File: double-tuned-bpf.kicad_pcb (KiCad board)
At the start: 2 copper layers, 92 x 71 mm, 96 parts, among them J1 PCB_SMA_EDGE, J2 PCB_SMA_EDGE, J3 Conn_01x03_Female, J4 Conn_01x03_Female, T1 6:31, T2 31:6

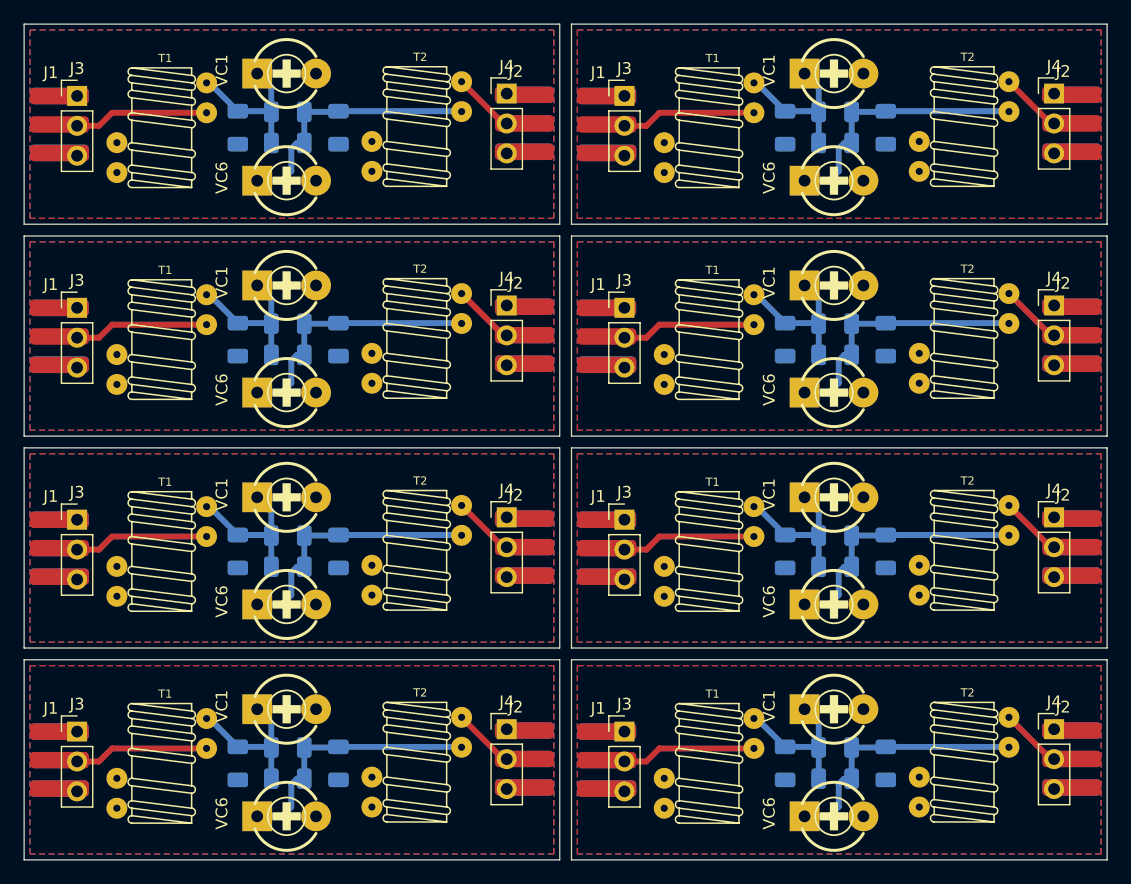
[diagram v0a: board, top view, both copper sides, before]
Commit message: gg
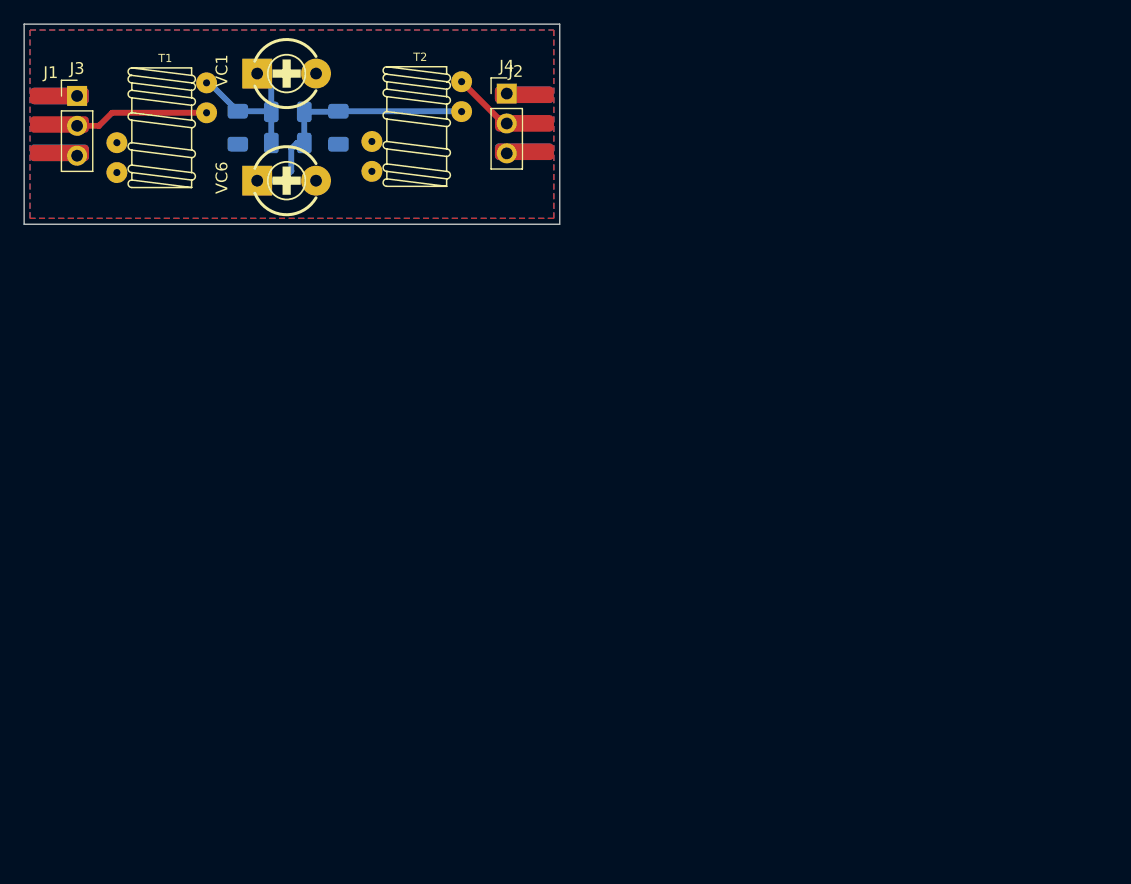
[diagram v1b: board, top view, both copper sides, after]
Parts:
- removed the C2 at (124.9, 133.8)
- removed the C2 at (171.4, 133.8)
- removed the C2 at (124.9, 151.8)
- removed the C2 at (171.4, 151.8)
- removed the C2 at (124.9, 115.8)
- removed the C2 at (171.4, 115.8)
- removed the C2 at (171.4, 97.8)
- removed the C3 at (173.4, 137.3)
- removed the C3 at (126.9, 137.3)
- removed the C3 at (173.4, 155.3)
- removed the C3 at (126.9, 155.3)
- removed the C3 at (173.4, 119.3)
- removed the C3 at (126.9, 119.3)
- removed the C3 at (173.4, 101.3)
- removed the C4 at (173.4, 134.7)
- removed the C4 at (126.9, 134.7)
- removed the C4 at (126.9, 152.7)
- removed the C4 at (173.4, 152.7)
- removed the C4 at (173.4, 116.7)
- removed the C4 at (126.9, 116.7)
- removed the C4 at (173.4, 98.7)
- removed the C5 at (133.4, 133.8)
- removed the C5 at (179.9, 133.8)
- removed the C5 at (133.4, 151.8)
- removed the C5 at (179.9, 151.8)
- removed the C5 at (133.4, 115.8)
- removed the C5 at (179.9, 115.8)
- removed the C5 at (179.9, 97.8)
- removed the J1 at (154.0, 146.4)
- removed the J1 at (107.5, 128.4)
- removed the J1 at (107.5, 146.4)
- removed the J1 at (154.0, 128.4)
- removed the J1 at (107.5, 110.4)
- removed the J1 at (154.0, 110.4)
- removed the J1 at (154.0, 92.4)
- removed the J2 at (193.5, 128.3)
- removed the J2 at (147.0, 128.3)
- removed the J2 at (193.5, 146.3)
- removed the J2 at (147.0, 146.3)
- removed the J2 at (193.5, 110.3)
- removed the J2 at (147.0, 110.3)
- removed the J2 at (193.5, 92.3)
- removed the J3 at (109.0, 131.1)
- removed the J3 at (155.5, 149.1)
- removed the J3 at (109.0, 149.1)
- removed the J3 at (155.5, 131.1)
- removed the J3 at (109.0, 113.1)
- removed the J3 at (155.5, 113.1)
- removed the J3 at (155.5, 95.1)
- removed the J4 at (192.0, 130.9)
- removed the J4 at (145.5, 130.9)
- removed the J4 at (192.0, 148.9)
- removed the J4 at (145.5, 148.9)
- removed the J4 at (192.0, 112.9)
- removed the J4 at (145.5, 112.9)
- removed the J4 at (192.0, 94.9)
- removed the T1 at (116.2, 126.8)
- removed the T1 at (162.7, 126.8)
- removed the T1 at (116.2, 144.8)
- removed the T1 at (162.7, 144.8)
- removed the T1 at (116.2, 108.8)
- removed the T1 at (162.7, 108.8)
- removed the T1 at (162.7, 90.8)
- removed the T2 at (137.9, 126.7)
- removed the T2 at (137.9, 144.7)
- removed the T2 at (184.4, 144.7)
- removed the T2 at (184.4, 126.7)
- removed the T2 at (137.9, 108.7)
- removed the T2 at (184.4, 108.7)
- removed the T2 at (184.4, 90.7)
- removed the VC1 at (120.3, 129.2)
- removed the VC1 at (166.8, 147.2)
- removed the VC1 at (120.3, 147.2)
- removed the VC1 at (166.8, 129.2)
- removed the VC1 at (120.3, 111.2)
- removed the VC1 at (166.8, 111.2)
- removed the VC1 at (166.8, 93.2)
- removed the VC6 at (120.3, 138.3)
- removed the VC6 at (166.8, 138.3)
- removed the VC6 at (166.8, 156.3)
- removed the VC6 at (120.3, 156.3)
- removed the VC6 at (120.3, 120.3)
- removed the VC6 at (166.8, 120.3)
- removed the VC6 at (166.8, 102.3)
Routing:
- net (no net): track 366.6 -> 0.00 mm
- removed copper zone on B.Cu, net (none)
- removed copper zone on F.Cu, net (none)
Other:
- board size 92 x 71 mm -> 45.5 x 17 mm
